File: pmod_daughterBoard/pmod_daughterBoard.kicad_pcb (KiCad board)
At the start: 2 copper layers, 36.8 x 68.6 mm, 17 parts, among them J1 Conn_02x04_Odd_Even, J11 Conn_02x06_Odd_Even, J2 Conn_02x04_Odd_Even, J3 Conn_Coaxial, J4 Conn_01x02_Male, Q1 N/A

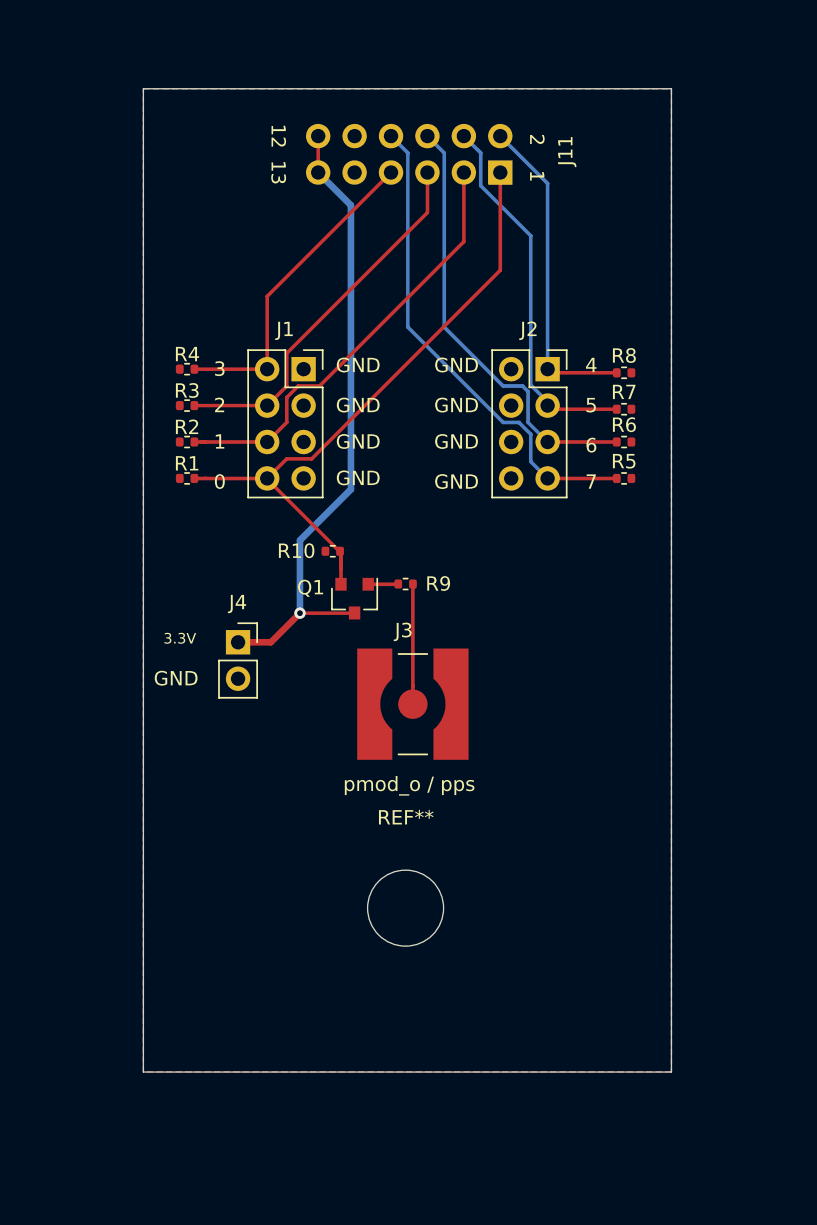
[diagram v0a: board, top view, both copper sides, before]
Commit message: update board
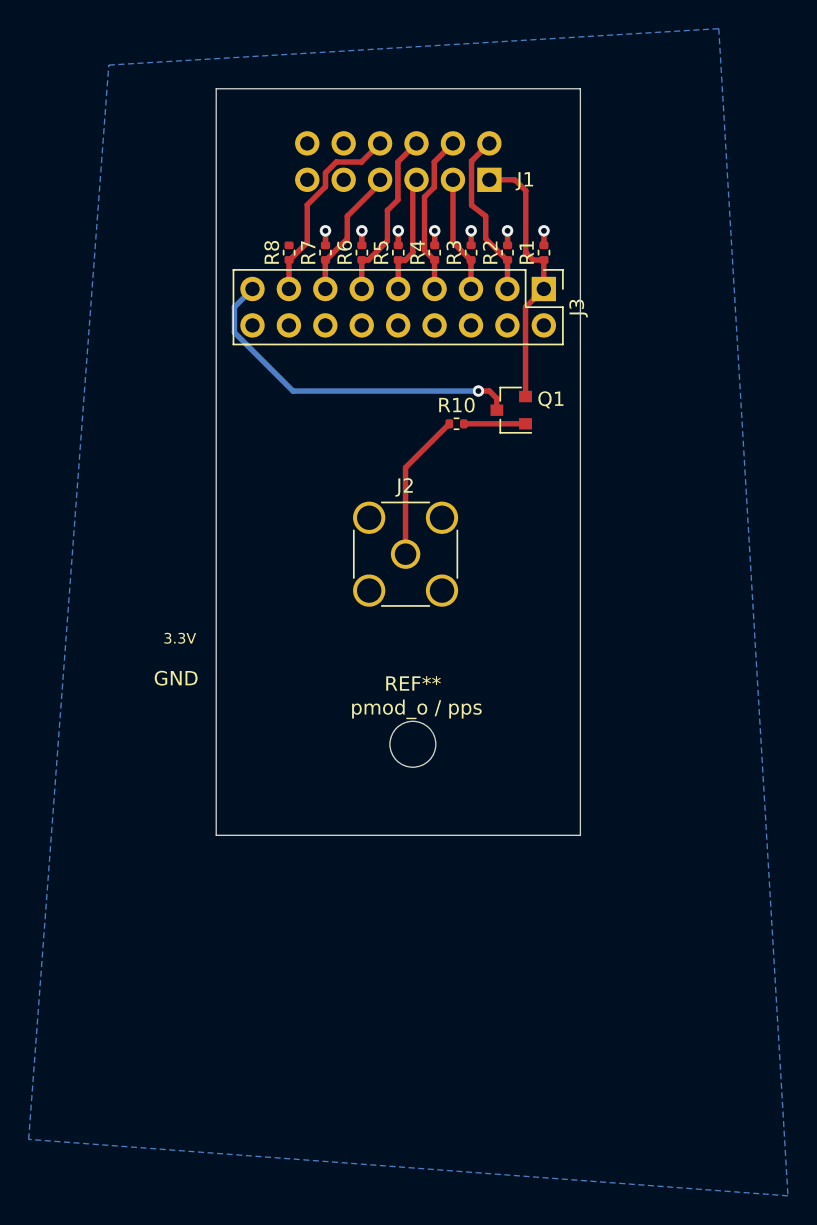
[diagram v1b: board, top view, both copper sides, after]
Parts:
- removed the J1 at (166.1, 56.4)
- removed the J2 at (183.1, 56.4)
- removed J4: Conn_01x02_Male, Connector_PinSocket_2.54mm:PinSocket_1x02_P2.54mm_Vertical
- removed the R10 at (168.1, 69.1)
- added J3: Conn_02x09_Odd_Even, Connector_PinHeader_2.54mm:PinHeader_2x09_P2.54mm_Vertical, F.Cu at (182.9, 50.8)
- J2: renamed from J3; footprint pmod_daughterBoard:LINX_CONSMA001-SMD-G-T -> Connector_Coaxial:SMA_Amphenol_132291-12_Vertical
- REF**: value MountingHole_5.3mm_M5 -> MountingHole_3.2mm_M3; footprint MountingHole:MountingHole_5.3mm_M5 -> MountingHole:MountingHole_3.2mm_M3
- moved R1 29.5 mm to (182.9, 48.3), turned to 90 degrees
- moved R2 26.0 mm to (180.3, 48.3), turned to 90 degrees
- moved R8 24.8 mm to (165.1, 48.3), turned to 90 degrees
- moved R7 23.5 mm to (167.6, 48.3), turned to 90 degrees
- moved R6 22.6 mm to (170.2, 48.3), turned to 90 degrees
- moved R3 22.5 mm to (177.8, 48.3), turned to 90 degrees
- moved R5 22.3 mm to (172.7, 48.3), turned to 90 degrees
- moved R4 19.1 mm to (175.3, 48.3), turned to 90 degrees
- moved Q1 17.1 mm to (180.6, 59.2), turned to 180 degrees
- moved R10 11.7 mm to (176.8, 60.2), turned to 0 degrees
- moved REF** 11.4 mm to (173.7, 82.5)
- moved J2 10.5 mm to (173.2, 69.3)
- moved J1 0.92 mm to (179.1, 43.2)
- renumbered J11 to J1, R9 to R10
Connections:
- net Net-(J1-Pad8) renamed GPIO1
- net Net-(J11-Pad6) renamed GPIO6
- J1 pad 2: Net-(J11-Pad2) -> GPIO2
- J1 pad 3: Net-(J1-Pad6) -> GPIO3
- J1 pad 4: Net-(J11-Pad4) -> GPIO4
- J1 pad 5: Net-(J1-Pad4) -> GPIO5
- J1 pad 7: Net-(J1-Pad2) -> GPIO7
- J1 pad 8: Net-(J11-Pad8) -> GPIO8
- R2 pad 1: Net-(J1-Pad6) -> GPIO2
- R3 pad 1: Net-(J1-Pad4) -> GPIO3
- R4 pad 1: Net-(J1-Pad2) -> GPIO4
- R5 pad 1: Net-(J11-Pad8) -> GPIO5
- R7 pad 1: Net-(J11-Pad4) -> GPIO7
- R8 pad 1: Net-(J11-Pad2) -> GPIO8
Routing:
- net Net-(J11-Pad8): track 33.9 -> 0.00 mm
- net Net-(J1-Pad6): track 30.7 -> 0.00 mm
- net GPIO1: track 45.2 -> 18.7 mm
- net Net-(J11-Pad4): track 26.1 -> 0.00 mm
- net Net-(J1-Pad4): track 26.0 -> 0.00 mm
- net Net-(J11-Pad2): track 22.6 -> 0.00 mm
- net Net-(J1-Pad2): track 22.4 -> 0.00 mm
- net +3V3: track 44.7 -> 24.6 mm
- net GPIO6: track 30.4 -> 12.0 mm
- net GPIO8: track 0.00 -> 13.8 mm
- net GPIO2: track 0.00 -> 11.8 mm
- net GPIO4: track 0.00 -> 11.3 mm
- net GPIO7: track 0.00 -> 9.22 mm
- net GPIO5: track 0.00 -> 8.44 mm
- net GPIO3: track 0.00 -> 8.14 mm
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- removed copper zone on F.Cu, net GND
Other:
- board size 36.8 x 68.6 mm -> 25.4 x 52.1 mm
- net class Default removed
- board text removed: "0"
- board text removed: "1"
- board text removed: "12"
- board text removed: "13"
- board text removed: "2"
- board text removed: "3"
- board text removed: "4"
- board text removed: "5"
- board text removed: "6"
- board text removed: "7"
